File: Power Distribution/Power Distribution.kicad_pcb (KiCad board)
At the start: 16 copper layers, 61 x 88 mm, 51 parts, among them IC3 PCM5102 Audio Stereo DAC

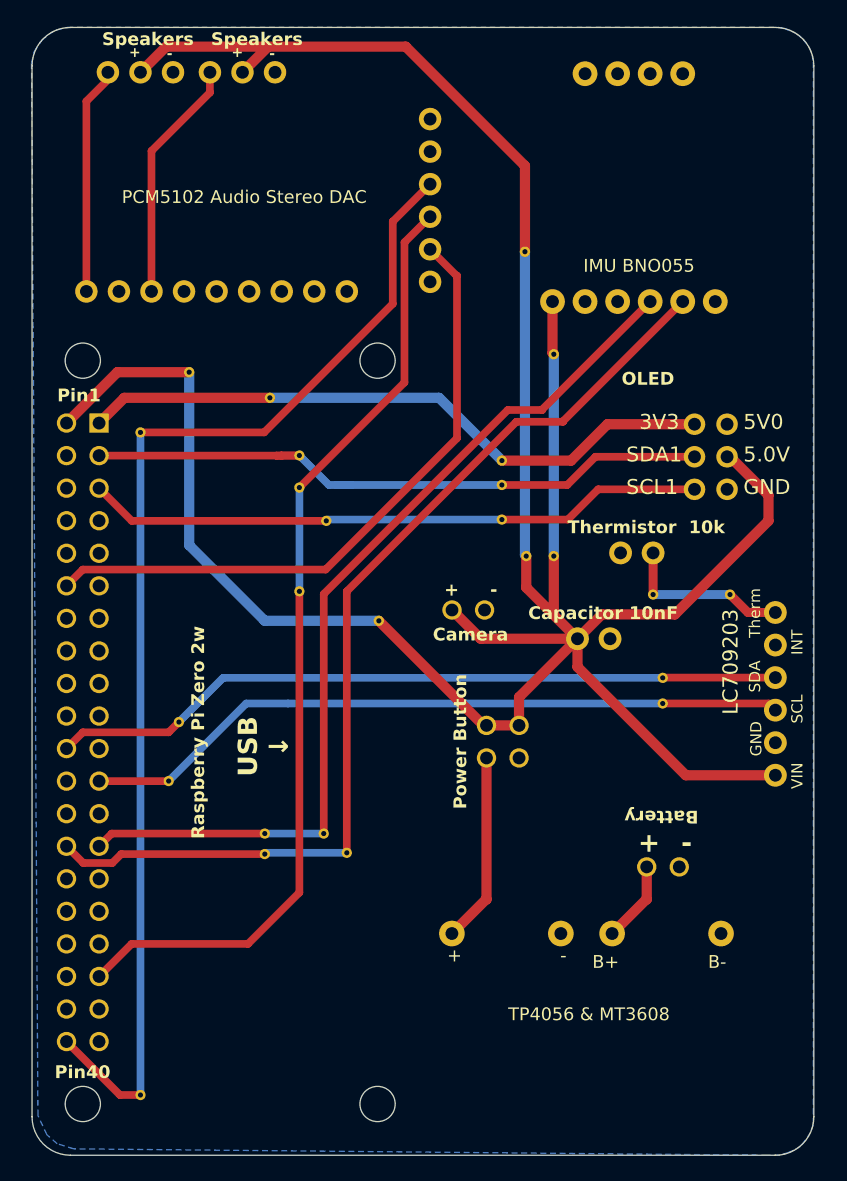
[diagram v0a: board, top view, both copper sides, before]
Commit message: PCB
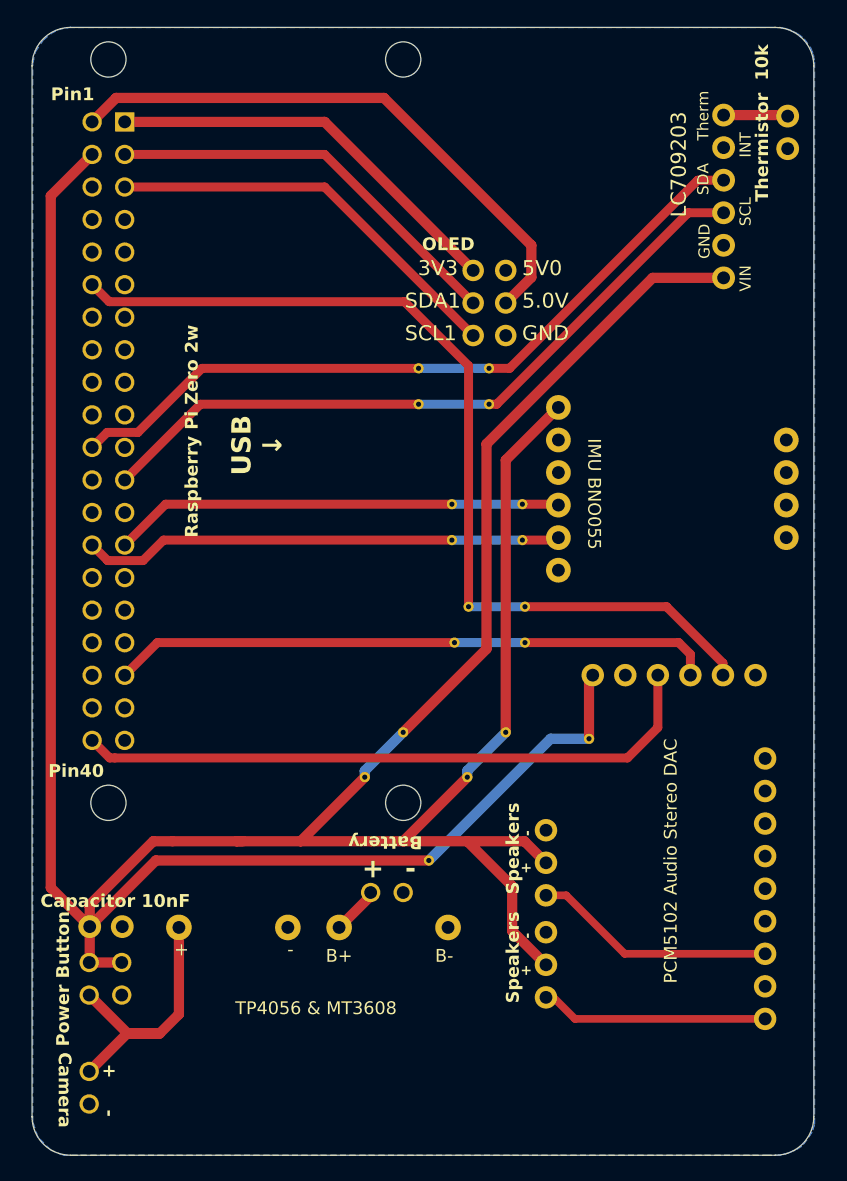
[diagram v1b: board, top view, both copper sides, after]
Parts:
- removed the ? at (248.2, 99.5)
- removed the ? at (225.7, 138.5)
- removed the ? at (219.8, 100.9)
- removed the ? at (225.7, 136.9)
- removed the ? at (256.0, 118.2)
- removed the ? at (244.2, 107.8)
- removed the ? at (228.4, 109.9)
- removed the ? at (230.5, 112.5)
- removed the ? at (232.1, 138.4)
- removed the ? at (218.2, 132.8)
- removed the ? at (226.1, 102.9)
- removed the ? at (216.0, 105.6)
- removed the ? at (230.3, 136.9)
- removed the ? at (248.2, 115.2)
- removed the ? at (234.6, 120.3)
- removed the ? at (246.0, 91.5)
- removed the ? at (246.1, 115.2)
- removed the ? at (228.4, 118.0)
- removed the ? at (219.0, 128.2)
- removed the ? at (216.0, 157.3)
- removed the ? at (228.4, 107.4)
- removed the ? at (244.2, 109.7)
- removed the ? at (244.2, 112.4)
- removed the ? at (262.0, 118.2)
- removed the ? at (256.8, 124.8)
- removed the ? at (256.8, 126.8)
- added ?: , , F.Cu at (241.5, 132.5)
- added ?: , , F.Cu at (243.2, 100.6)
- added ?: , , F.Cu at (243.2, 103.4)
- added ?: , , F.Cu at (233.5, 132.5)
- added ?: , , F.Cu at (244.5, 129.0)
- added ?: , , F.Cu at (246.0, 122.0)
- added ?: , , F.Cu at (251.0, 129.5)
- added ?: , , F.Cu at (245.8, 111.2)
- added ?: , , F.Cu at (238.5, 139.0)
- added ?: , , F.Cu at (245.8, 114.0)
- added ?: , , F.Cu at (240.3, 111.2)
- added ?: , , F.Cu at (241.6, 119.2)
- added ?: , , F.Cu at (240.5, 122.0)
- added ?: , , F.Cu at (246.0, 119.2)
- added ?: , , F.Cu at (237.7, 100.6)
- added ?: , , F.Cu at (236.5, 129.0)
- added ?: , , F.Cu at (237.7, 103.4)
- added ?: , , F.Cu at (240.3, 114.0)
- moved ? 79.9 mm to (247.6, 149.7), turned to 180 degrees
- moved ? 76.5 mm to (247.6, 147.1), turned to 180 degrees
- moved ? 73.1 mm to (247.6, 144.6), turned to 180 degrees
- moved ? 69.4 mm to (247.6, 141.7), turned to 180 degrees
- moved ? 66.1 mm to (247.6, 139.2), turned to 180 degrees
- moved ? 62.8 mm to (247.6, 136.6), turned to 180 degrees
- moved ? 49.4 mm to (212.0, 158.0), turned to 0 degrees
- moved IC3 48.9 mm to (264.7, 131.0), turned to -90 degrees
- moved ? 45.8 mm to (212.0, 155.5), turned to 0 degrees
- moved ? 44.2 mm to (212.0, 144.2)
- moved ? 44.2 mm to (214.6, 144.2)
- moved REF** 39.0 mm to (261.5, 87.2)
- moved ? 36.1 mm to (214.5, 149.5)
- moved ? 36.1 mm to (212.0, 149.5)
- moved ? 36.1 mm to (214.5, 147.0)
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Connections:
- ? pad 2: (no net) -> GND (x3)
- ? pad 3: (no net) -> GND (x3)
- ? pad 2: (no net) -> 5V (x3)
- ? pad 4: (no net) -> 5V
- ? pad 1: (no net) -> 5V
- ? pad 1: (no net) -> GND
- IC3 pad 1: (no net) -> 5V
- IC3 pad 12: (no net) -> GND
- IC3 pad 14: (no net) -> GND
- IC3 pad 2: (no net) -> GND
- IC3 pad 4: (no net) -> Signals
- IC3 pad 5: (no net) -> Signals
- REF** pad 1: (no net) -> 5V (x2)
- REF** pad 2: (no net) -> GND
- REF** pad 4: (no net) -> 5V (x2)
- REF** pad 6: (no net) -> GND (x2)
- REF** pad 3: (no net) -> GND
- REF** pad 12: (no net) -> Signals
- REF** pad 14: (no net) -> GND
- REF** pad 2: (no net) -> 5V
- REF** pad 20: (no net) -> GND
- REF** pad 22: (no net) -> Signals
- REF** pad 23: (no net) -> Signals
- REF** pad 25: (no net) -> GND
- REF** pad 27: (no net) -> Signals
- REF** pad 28: (no net) -> Signals
- REF** pad 3: (no net) -> Signals
- REF** pad 30: (no net) -> GND
- REF** pad 34: (no net) -> GND
- REF** pad 39: (no net) -> GND
- REF** pad 5: (no net) -> Signals
- REF** pad 9: (no net) -> GND
- TP4056 & MT3608 pad 2: (no net) -> GND
- TP4056 & MT3608 pad 4: (no net) -> GND
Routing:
- net (no net): track 926.9 -> 149.2 mm
- net Signals: track 0.00 -> 370.7 mm
- net 5V: track 0.00 -> 316.0 mm
- added copper zone on B.Cu, net GND
- removed copper zone on B.Cu, net (none)

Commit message: PCB
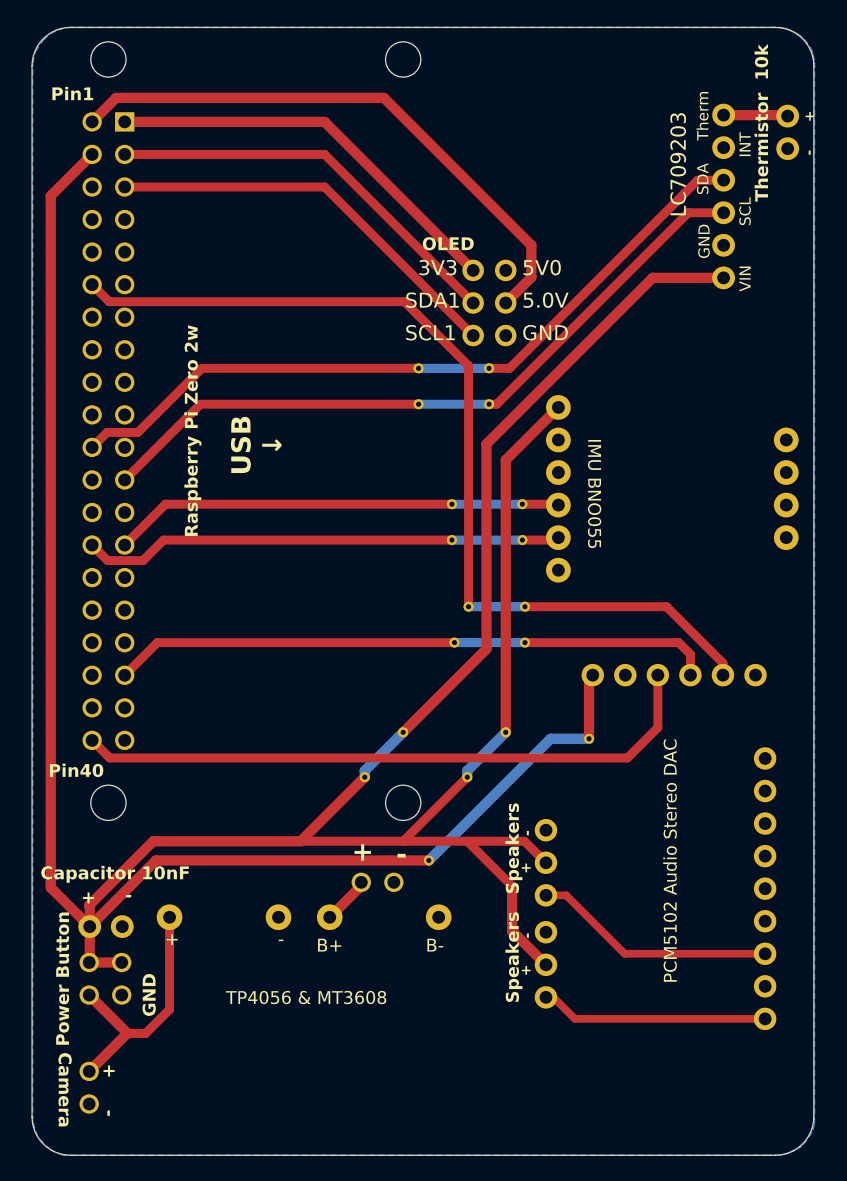
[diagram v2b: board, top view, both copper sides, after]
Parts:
- moved TP4056 & MT3608 1.08 mm to (228.0, 147.7)
- moved ? 1.08 mm to (233.2, 140.7)
- moved ? 1.08 mm to (235.8, 140.7)
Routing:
- net (no net): track 149.2 -> 146.5 mm
- net 5V: track 316.0 -> 315.5 mm
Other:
- board text removed: "Battery"
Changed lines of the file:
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@@
 	(footprint "ChargingBoardTP4056:Charging Board TP4056"
 		(layer "F.Cu")
-		(at 228.7 148.525)
+		(at 227.97 147.73)
 		(property "Reference" "TP4056 & MT3608"
 			(at 1 2 0)
@@
 	(footprint ""
 		(layer "F.Cu")
-		(at 236.5 141.5 90)
+		(at 235.77 140.705 90)
 		(property "Reference" ""
 			(at 0 0 90)
@@
 	(footprint ""
 		(layer "F.Cu")
-		(at 233.96 141.5 90)
+		(at 233.23 140.705 90)
 		(property "Reference" ""
 			(at 0 0 90)
@@
 		(layer "Edge.Cuts")
 	)
-	(gr_text "Pin40"
-		(at 208.8 132.6 0)
+	(gr_text "+"
+		(at 211.4 142.5 270)
 		(layer "F.SilkS")
 		(effects
@@
 				(bold yes)
 			)
-			(justify left bottom)
+			(justify left bottom mirror)
 		)
 	)
-	(gr_text "Battery"
-		(at 238 137 180)
+	(gr_text "Pin40"
+		(at 208.8 132.6 0)
 		(layer "F.SilkS")
 		(effects
@@
 	)
 	(gr_text "Capacitor 10nF"
-		(at 214.04 142.16 0)
+		(at 214.04 140 0)
 		(layer "F.SilkS")
 		(effects
@@
 		)
 	)
+	(gr_text "-"
+		(at 267.8 84 270)
+		(layer "F.SilkS")
+		(effects
+			(font
+				(size 0.8 0.8)
+				(thickness 0.16)
+				(bold yes)
+			)
+			(justify left bottom mirror)
+		)
+	)
 	(gr_text "SCL"
 		(at 263.207 88.373 90)
@@
 		)
 	)
+	(gr_text "-"
+		(at 215.35 142.3 0)
+		(layer "F.SilkS")
+		(effects
+			(font
+				(size 1 1)
+				(thickness 0.25)
+				(bold yes)
+			)
+			(justify left bottom mirror)
+		)
+	)
 	(gr_text "Camera"
 		(at 209.5 153.96 270)
@@
 		)
 	)
+	(gr_text "+"
+		(at 267.8 81.4 270)
+		(layer "F.SilkS")
+		(effects
+			(font
+				(size 0.8 0.8)
+				(thickness 0.16)
+				(bold yes)
+			)
+			(justify left bottom mirror)
+		)
+	)
 	(gr_text "LC709203"
 		(at 258 84.69 90)
@@
 	)
 	(gr_text "-\n"
-		(at 237.5 140.5 0)
+		(at 236.8 139.4 0)
 		(layer "F.SilkS")
 		(effects
@@
 		)
 	)
+	(gr_text "GND"
+		(at 217.3 151.2 90)
+		(layer "F.SilkS")
+		(effects
+			(font
+				(size 1 1)
+				(thickness 0.25)
+				(bold yes)
+			)
+			(justify left bottom)
+		)
+	)
 	(gr_text "Speakers\n"
 		(at 245.64 141.64 90)
@@
 	)
 	(gr_text "+\n"
-		(at 235 140.5 0)
+		(at 234.2 139.2 0)
 		(layer "F.SilkS")
 		(effects
@@
 	)
 	(segment
-		(start 254 131)
-		(end 214 131)
+		(start 214.77 81.37)
+		(end 230.37 81.37)
+		(width 0.8)
+		(layer "F.Cu")
+		(net 0)
+	)
+	(segment
+		(start 218.27 143.43)
+		(end 218.27 150.63)
 		(width 0.7)
 		(layer "F.Cu")
@@
 	)
 	(segment
-		(start 214.77 81.37)
-		(end 230.37 81.37)
-		(width 0.8)
+		(start 254 131)
+		(end 256.37 128.63)
+		(width 0.7)
 		(layer "F.Cu")
 		(net 0)
 	)
 	(segment
-		(start 214.96 152.5)
-		(end 217.5 152.5)
-		(width 0.8)
+		(start 212.23 129.63)
+		(end 213.6 131)
+		(width 0.7)
 		(layer "F.Cu")
 		(net 0)
@@
 	)
 	(segment
-		(start 231.5 144.225)
-		(end 233.96 141.765)
+		(start 230.77 143.43)
+		(end 233.23 140.97)
 		(width 0.8)
 		(layer "F.Cu")
@@
 	)
 	(segment
-		(start 256.37 124.54)
-		(end 256.37 128.63)
-		(width 0.7)
+		(start 247.64 141.72)
+		(end 249.22 141.72)
+		(width 0.6)
 		(layer "F.Cu")
 		(net 0)
 	)
 	(segment
-		(start 256.37 128.63)
+		(start 213.6 131)
 		(end 254 131)
 		(width 0.7)
@@
 	)
 	(segment
-		(start 247.64 141.72)
-		(end 249.22 141.72)
-		(width 0.6)
-		(layer "F.Cu")
-		(net 0)
-	)
-	(segment
-		(start 219 151)
-		(end 219 144.225)
-		(width 0.8)
+		(start 256.37 128.63)
+		(end 256.37 124.54)
+		(width 0.7)
 		(layer "F.Cu")
 		(net 0)
@@
 	)
 	(segment
-		(start 216.5 152.5)
-		(end 217.5 152.5)
-		(width 0.8)
-		(layer "F.Cu")
-		(net 0)
-	)
-	(segment
-		(start 253.78 146.28)
-		(end 264.74 146.28)
-		(width 0.6)
+		(start 218.27 150.63)
+		(end 216.4 152.5)
+		(width 0.7)
 		(layer "F.Cu")
 		(net 0)
 	)
 	(segment
-		(start 214 131)
-		(end 213.6 131)
+		(start 215 152.5)
+		(end 216.4 152.5)
 		(width 0.7)
 		(layer "F.Cu")
@@
 	)
 	(segment
-		(start 233.96 141.765)
-		(end 233.96 141.5)
-		(width 0.8)
+		(start 253.78 146.28)
+		(end 264.74 146.28)
+		(width 0.6)
 		(layer "F.Cu")
 		(net 0)
 	)
 	(segment
-		(start 217.5 152.5)
-		(end 219 151)
+		(start 233.23 140.97)
+		(end 233.23 140.705)
 		(width 0.8)
 		(layer "F.Cu")
@@
 	)
 	(segment
-		(start 213.6 131)
-		(end 212.23 129.63)
-		(width 0.7)
-		(layer "F.Cu")
-		(net 0)
-	)
-	(segment
-		(start 215 152.5)
-		(end 216.5 152.5)
-		(width 0.8)
-		(layer "F.Cu")
-		(net 0)
-	)
-	(segment
 		(start 249.9 151.36)
 		(end 264.74 151.36)
@@
 	(segment
 		(start 228.5 137.5)
-		(end 234 137.5)
-		(width 0.8)
-		(layer "F.Cu")
-		(net 2)
-	)
-	(segment
-		(start 236.5 137.5)
-		(end 241.5 132.5)
-		(width 0.8)
-		(layer "F.Cu")
-		(net 2)
-	)
-	(segment
-		(start 241.5 137.5)
-		(end 245.96 137.5)
-		(width 0.8)
+		(end 236.5 137.5)
+		(width 0.7)
 		(layer "F.Cu")
 		(net 2)
@@
 	)
 	(segment
-		(start 223.5 137.5)
-		(end 224 137.5)
-		(width 0.8)
-		(layer "F.Cu")
-		(net 2)
-	)
-	(segment
 		(start 212.04 144.16)
 		(end 212.04 146.92)
@@
 	(segment
 		(start 217 137.5)
-		(end 218.5 137.5)
+		(end 228.5 137.5)
 		(width 0.8)
 		(layer "F.Cu")
@@
 	)
 	(segment
+		(start 245.96 137.5)
+		(end 247.64 139.18)
+		(width 0.7)
+		(layer "F.Cu")
+		(net 2)
+	)
+	(segment
 		(start 243 106.5)
 		(end 255.96 93.54)
@@
 	)
 	(segment
-		(start 236.5 137.5)
+		(start 245 141)
 		(end 241.5 137.5)
-		(width 0.8)
+		(width 0.7)
 		(layer "F.Cu")
 		(net 2)
@@
 	)
 	(segment
-		(start 217.2 139)
-		(end 238.5 139)
-		(width 0.8)
+		(start 241.5 137.5)
+		(end 245.96 137.5)
+		(width 0.7)
 		(layer "F.Cu")
 		(net 2)
 	)
 	(segment
-		(start 243 122.5)
-		(end 243 106.5)
-		(width 0.8)
+		(start 236.5 137.5)
+		(end 241.5 132.5)
+		(width 0.7)
 		(layer "F.Cu")
 		(net 2)
 	)
 	(segment
-		(start 234 137.5)
+		(start 241.5 137.5)
 		(end 236.5 137.5)
-		(width 0.8)
+		(width 0.7)
 		(layer "F.Cu")
 		(net 2)
 	)
 	(segment
-		(start 209 87.14)
-		(end 212.23 83.91)
+		(start 217.2 139)
+		(end 238.5 139)
 		(width 0.8)
 		(layer "F.Cu")
@@
 	)
 	(segment
-		(start 251 129.5)
-		(end 251 124.83)
+		(start 243 122.5)
+		(end 243 106.5)
 		(width 0.8)
 		(layer "F.Cu")
@@
 	)
 	(segment
-		(start 218.5 137.5)
-		(end 223.5 137.5)
+		(start 209 87.14)
+		(end 212.23 83.91)
 		(width 0.8)
 		(layer "F.Cu")
@@
 	)
 	(segment
-		(start 212.04 144.16)
-		(end 209 141.12)
+		(start 251 129.5)
+		(end 251 124.83)
 		(width 0.8)
 		(layer "F.Cu")
@@
 	)
 	(segment
-		(start 248.61 103.65)
-		(end 244.5 107.76)
+		(start 212.04 144.16)
+		(end 209 141.12)
 		(width 0.8)
 		(layer "F.Cu")
@@
 	)
 	(segment
-		(start 223.5 137.5)
-		(end 228.5 137.5)
+		(start 248.61 103.65)
+		(end 244.5 107.76)
 		(width 0.8)
 		(layer "F.Cu")
@@
 	)
 	(segment
-		(start 245.96 137.5)
-		(end 247.64 139.18)
-		(width 0.8)
-		(layer "F.Cu")
-		(net 2)
-	)
-	(segment
 		(start 233.5 132.5)
 		(end 228.5 137.5)
 		(width 0.8)
 		(layer "F.Cu")
-		(net 2)
-	)
-	(segment
-		(start 241.5 137.5)
-		(end 245 141)
-		(width 0.8)
-		(layer "F.Cu")
